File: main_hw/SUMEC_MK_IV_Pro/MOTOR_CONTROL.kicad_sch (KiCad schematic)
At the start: 16 parts, among them IC2 DRV8874PWPR, IC3 DRV8874PWPR

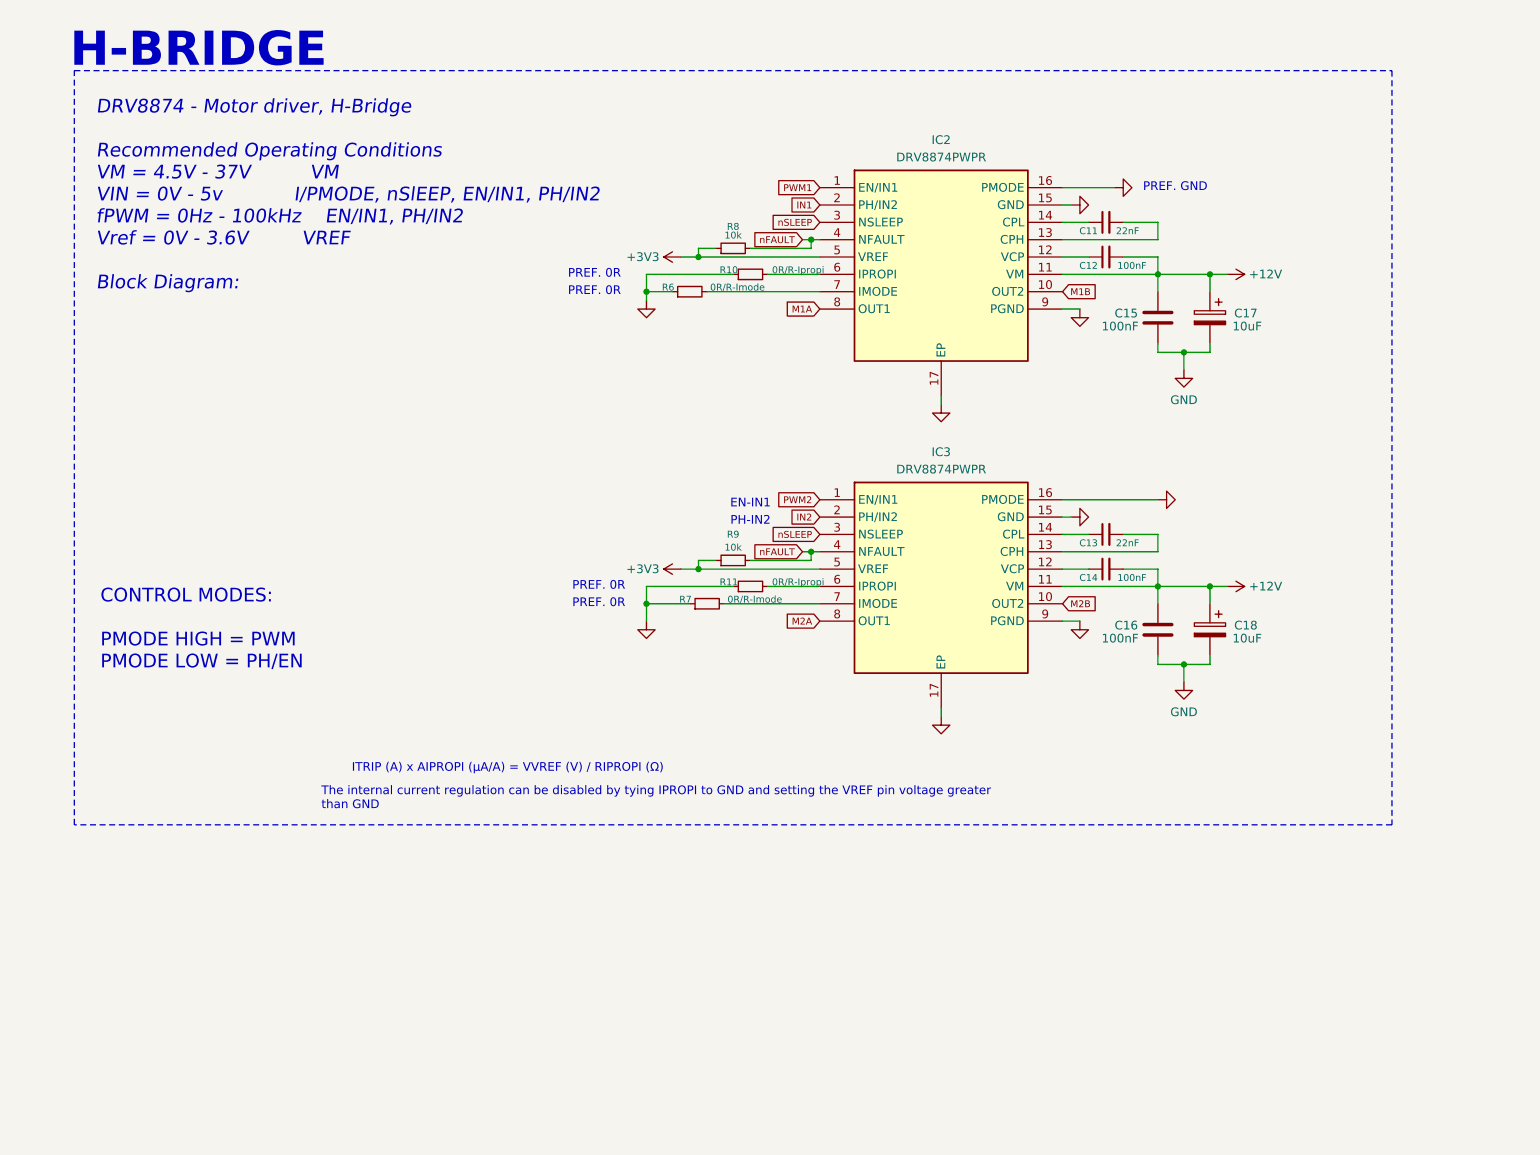
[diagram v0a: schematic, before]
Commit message: Force push
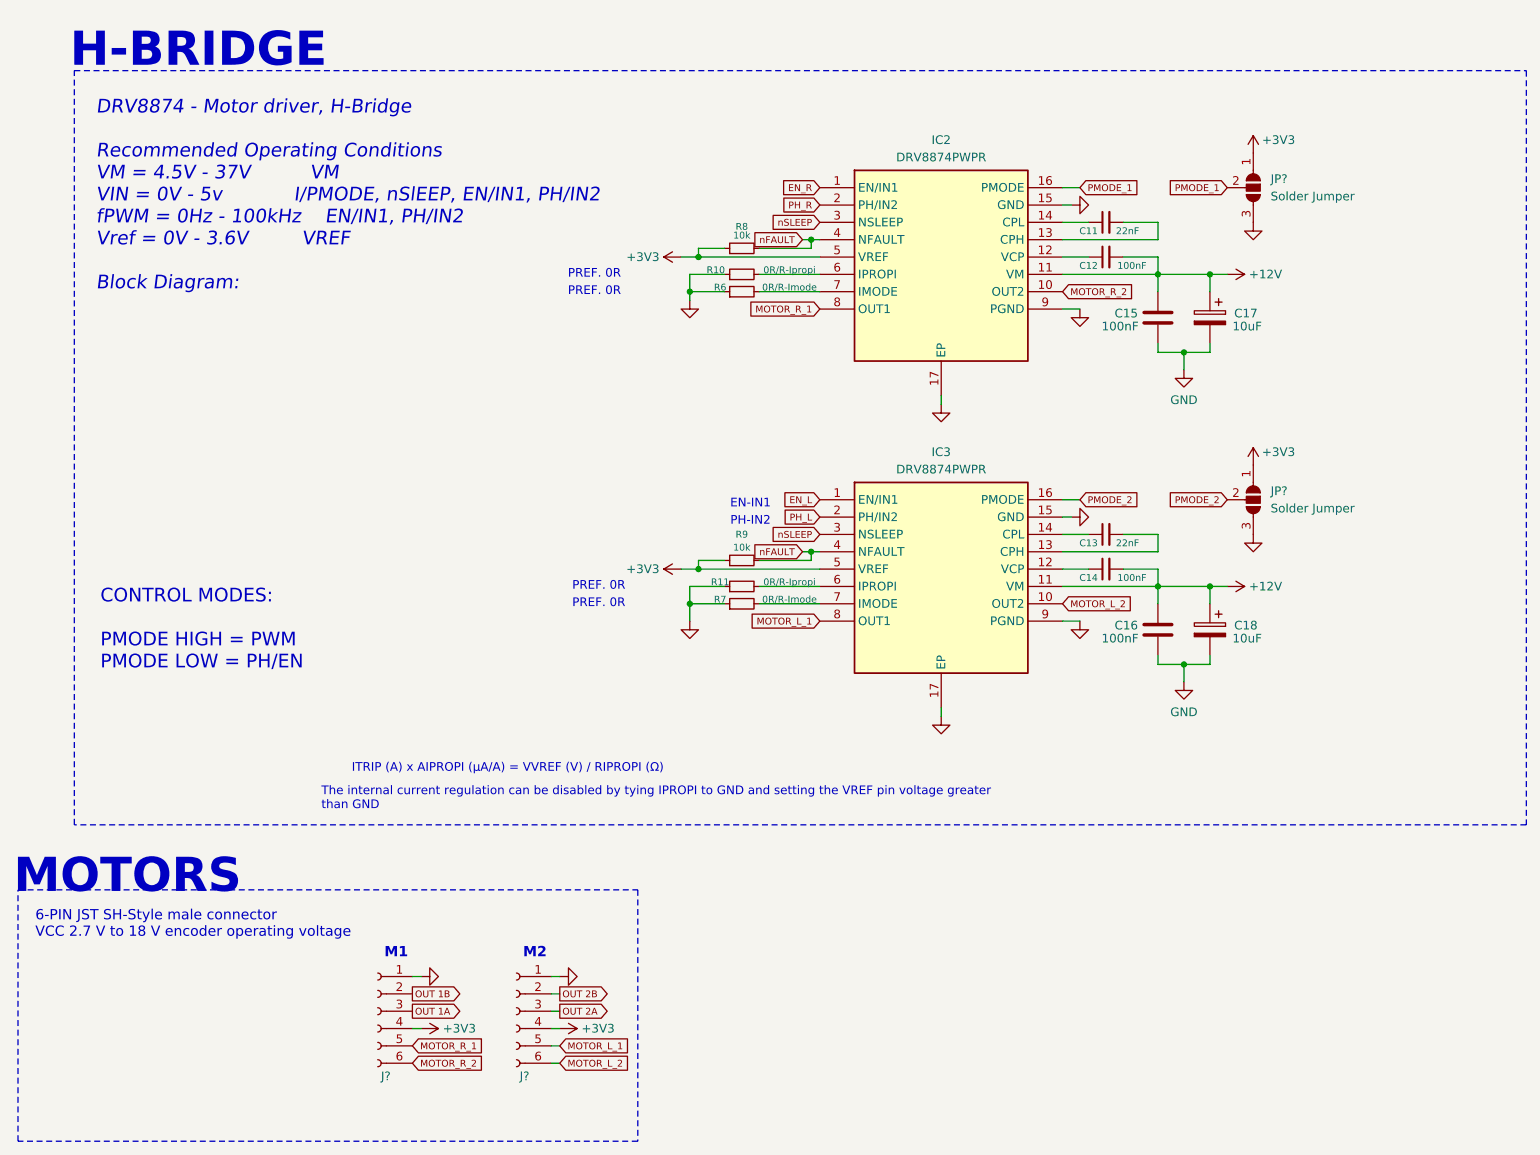
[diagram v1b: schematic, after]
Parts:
- added J? (x2): Conn_01x06_Socket, Connector_JST:JST_SH_BM06B-SRSS-TB_1x06-1MP_P1.00mm_Vertical, symbol Connector:Conn_01x06_Socket
- added JP? (x2): Solder Jumper, symbol Jumper:SolderJumper_3_Open
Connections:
- net +3V3: now also J?.4 (Pin_4), J?.4 (Pin_4), JP?.1 (A), JP?.1 (A)
- net GND: now also J?.1 (Pin_1), J?.1 (Pin_1), JP?.3 (B), JP?.3 (B); no longer IC2.16 (PMODE), IC3.16 (PMODE)
- net IN1 renamed PH_R
- net IN2 renamed PH_L
- net M1A renamed MOTOR_R_1
- net MOTOR_R_1: now also J?.5 (Pin_5)
- net M1B renamed MOTOR_R_2
- net MOTOR_R_2: now also J?.6 (Pin_6)
- net M2A renamed MOTOR_L_1
- net MOTOR_L_1: now also J?.5 (Pin_5)
- net M2B renamed MOTOR_L_2
- net MOTOR_L_2: now also J?.6 (Pin_6)
- net PWM1 renamed EN_R
- net PWM2 renamed EN_L
- new net OUT 1A: J?.3 (Pin_3)
- new net OUT 1B: J?.2 (Pin_2)
- new net OUT 2A: J?.3 (Pin_3)
- new net OUT 2B: J?.2 (Pin_2)
- new net PMODE_1: IC2.16 (PMODE), JP?.2 (C)
- new net PMODE_2: IC3.16 (PMODE), JP?.2 (C)
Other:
- note added: "6-PIN JST SH-Style male connector VCC 2.7 V to 18 V encoder operating voltage"
- note added: "M1"
- note added: "M2"
- note added: "MOTORS"
- note removed: "PREF. GND"
- moved on the sheet: R10, R11, R6, R7, R8, R9
